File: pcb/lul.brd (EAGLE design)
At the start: 90 x 96 mm, 88 parts, among them IC1 STM32F072C8T6, IC2 REG1117, IC3 74LVC1G125DBV, U1 UG-2864HSWEG01, X1 USB-MICROB

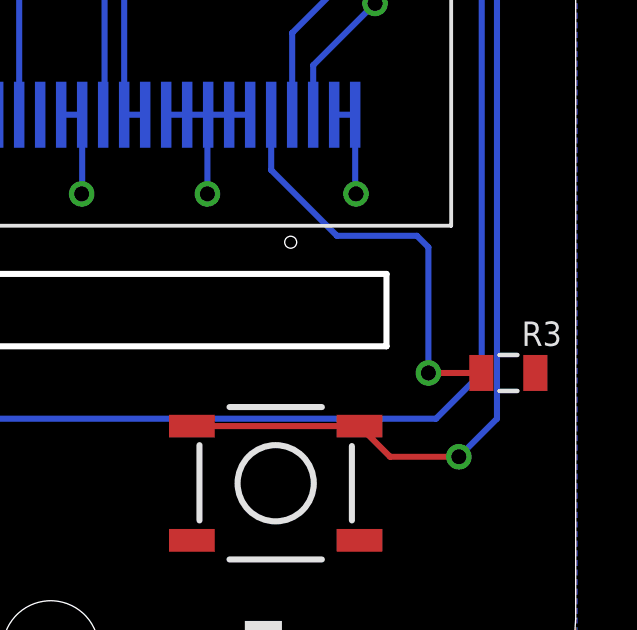
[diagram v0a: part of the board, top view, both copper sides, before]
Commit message: started working on board firmware
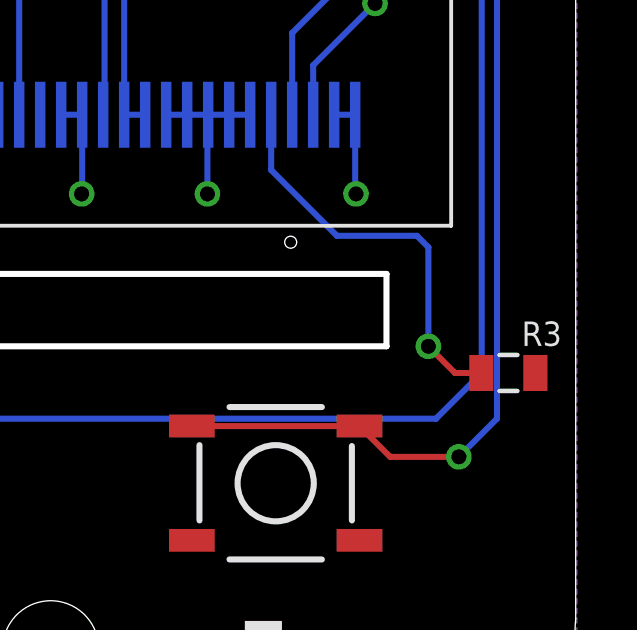
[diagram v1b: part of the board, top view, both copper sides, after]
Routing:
- net N$3: track 14.1 -> 13.6 mm
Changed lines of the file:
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@@
 <layer number="14" name="Route14" color="1" fill="6" visible="no" active="no"/>
 <layer number="15" name="Route15" color="4" fill="6" visible="no" active="no"/>
-<layer number="16" name="Bottom" color="1" fill="1" visible="yes" active="yes"/>
+<layer number="16" name="Bottom" color="1" fill="1" visible="no" active="yes"/>
 <layer number="17" name="Pads" color="2" fill="1" visible="yes" active="yes"/>
 <layer number="18" name="Vias" color="2" fill="1" visible="yes" active="yes"/>
@@
 <layer number="20" name="Dimension" color="15" fill="1" visible="yes" active="yes"/>
 <layer number="21" name="tPlace" color="7" fill="1" visible="yes" active="yes"/>
-<layer number="22" name="bPlace" color="7" fill="1" visible="yes" active="yes"/>
+<layer number="22" name="bPlace" color="7" fill="1" visible="no" active="yes"/>
 <layer number="23" name="tOrigins" color="15" fill="1" visible="yes" active="yes"/>
-<layer number="24" name="bOrigins" color="15" fill="1" visible="yes" active="yes"/>
+<layer number="24" name="bOrigins" color="15" fill="1" visible="no" active="yes"/>
 <layer number="25" name="tNames" color="7" fill="1" visible="yes" active="yes"/>
-<layer number="26" name="bNames" color="7" fill="1" visible="yes" active="yes"/>
-<layer number="27" name="tValues" color="7" fill="1" visible="yes" active="yes"/>
-<layer number="28" name="bValues" color="7" fill="1" visible="yes" active="yes"/>
+<layer number="26" name="bNames" color="7" fill="1" visible="no" active="yes"/>
+<layer number="27" name="tValues" color="7" fill="1" visible="no" active="yes"/>
+<layer number="28" name="bValues" color="7" fill="1" visible="no" active="yes"/>
 <layer number="29" name="tStop" color="7" fill="3" visible="no" active="yes"/>
 <layer number="30" name="bStop" color="7" fill="6" visible="no" active="yes"/>
@@
 <layer number="37" name="tTest" color="7" fill="1" visible="no" active="yes"/>
 <layer number="38" name="bTest" color="7" fill="1" visible="no" active="yes"/>
-<layer number="39" name="tKeepout" color="4" fill="11" visible="no" active="yes"/>
+<layer number="39" name="tKeepout" color="4" fill="11" visible="yes" active="yes"/>
 <layer number="40" name="bKeepout" color="1" fill="11" visible="no" active="yes"/>
-<layer number="41" name="tRestrict" color="4" fill="10" visible="no" active="yes"/>
+<layer number="41" name="tRestrict" color="4" fill="10" visible="yes" active="yes"/>
 <layer number="42" name="bRestrict" color="1" fill="10" visible="no" active="yes"/>
 <layer number="43" name="vRestrict" color="2" fill="10" visible="no" active="yes"/>
 <layer number="44" name="Drills" color="7" fill="1" visible="no" active="yes"/>
-<layer number="45" name="Holes" color="7" fill="1" visible="no" active="yes"/>
-<layer number="46" name="Milling" color="3" fill="1" visible="no" active="yes"/>
+<layer number="45" name="Holes" color="7" fill="1" visible="yes" active="yes"/>
+<layer number="46" name="Milling" color="3" fill="1" visible="yes" active="yes"/>
 <layer number="47" name="Measures" color="7" fill="1" visible="no" active="yes"/>
 <layer number="48" name="Document" color="7" fill="1" visible="no" active="yes"/>
 <layer number="49" name="Reference" color="7" fill="1" visible="no" active="yes"/>
 <layer number="50" name="dxf" color="7" fill="1" visible="no" active="no"/>
-<layer number="51" name="tDocu" color="7" fill="1" visible="no" active="yes"/>
+<layer number="51" name="tDocu" color="7" fill="1" visible="yes" active="yes"/>
 <layer number="52" name="bDocu" color="7" fill="1" visible="no" active="yes"/>
 <layer number="53" name="tGND_GNDA" color="7" fill="9" visible="no" active="no"/>
@@
 <contactref element="U1" pad="26"/>
 <contactref element="R3" pad="2"/>
-<via x="85.09" y="12.192" extent="1-16" drill="0.5"/>
+<via x="85.09" y="13.081" extent="1-16" drill="0.5"/>
 <wire x1="79.85" y1="18.956" x2="82.042" y2="16.764" width="0.2032" layer="16"/>
 <wire x1="82.042" y1="16.764" x2="84.709" y2="16.764" width="0.2032" layer="16"/>
 <wire x1="84.709" y1="16.764" x2="85.09" y2="16.383" width="0.2032" layer="16"/>
-<wire x1="85.09" y1="16.383" x2="85.09" y2="12.192" width="0.2032" layer="16"/>
+<wire x1="85.09" y1="16.383" x2="85.09" y2="13.081" width="0.2032" layer="16"/>
 <wire x1="79.85" y1="20.8" x2="79.85" y2="18.956" width="0.2032" layer="16"/>
-<wire x1="86.857" y1="12.192" x2="85.09" y2="12.192" width="0.2032" layer="1"/>
+<wire x1="86.857" y1="12.192" x2="85.979" y2="12.192" width="0.2032" layer="1"/>
+<wire x1="85.979" y1="12.192" x2="85.09" y2="13.081" width="0.2032" layer="1"/>
 </signal>
 <signal name="N$4">

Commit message: RTOS working start
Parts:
- C3, C4, C6, C7: value 1uF -> 2.2uF
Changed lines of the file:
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@@
 <attribute name="NAME" x="89.535" y="13.9065" size="0.8128" layer="25" rot="R180"/>
 </element>
-<element name="C3" library="clock" package="0805@1" value="1uF" x="66.294" y="40.005" smashed="yes" rot="R180">
+<element name="C3" library="clock" package="0805@1" value="2.2uF" x="66.294" y="40.005" smashed="yes" rot="R180">
 <attribute name="NAME" x="67.945" y="39.0525" size="0.8128" layer="25" rot="R180"/>
 </element>
-<element name="C4" library="clock" package="0805@1" value="1uF" x="69.596" y="40.005" smashed="yes" rot="R180">
+<element name="C4" library="clock" package="0805@1" value="2.2uF" x="69.596" y="40.005" smashed="yes" rot="R180">
 <attribute name="NAME" x="71.247" y="39.0525" size="0.8128" layer="25" rot="R180"/>
 </element>
@@
 <attribute name="NAME" x="88.265" y="38.9255" size="0.8128" layer="25" rot="R180"/>
 </element>
-<element name="C7" library="clock" package="0805@1" value="1uF" x="58.928" y="12.192" smashed="yes">
+<element name="C7" library="clock" package="0805@1" value="2.2uF" x="58.928" y="12.192" smashed="yes">
 <attribute name="NAME" x="57.531" y="13.2715" size="0.8128" layer="25"/>
 </element>
@@
 <attribute name="NAME" x="84.836" y="38.9255" size="0.8128" layer="25" rot="R180"/>
 </element>
-<element name="C6" library="clock" package="0805@1" value="1uF" x="58.928" y="10.033" smashed="yes">
+<element name="C6" library="clock" package="0805@1" value="2.2uF" x="58.928" y="10.033" smashed="yes">
 <attribute name="NAME" x="58.293" y="8.1915" size="0.8128" layer="25"/>
 </element>
